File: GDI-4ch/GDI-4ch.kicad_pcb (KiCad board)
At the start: 4 copper layers, 380.4 x 234.8 mm, 165 parts, among them J14 CONN_01X03, J15 CONN_01X01, J3 CONN_02X08, J4 CONN_02X08, J7 CONN_01X03, P1 368255-2, Q1 BUK9230-100B, Q10 BUK9230-100B, Q11 BUK9230-100B, Q12 BUK9230-100B, Q2 BUK9230-100B, Q3 BUK9230-100B, Q4 BUK9230-100B, Q5 BUK9230-100B, Q6 BUK9230-100B, Q7 BUK9230-100B, Q8 BUK9230-100B, Q9 BUK9230-100B, U1 MC33816, Y2 1MHz

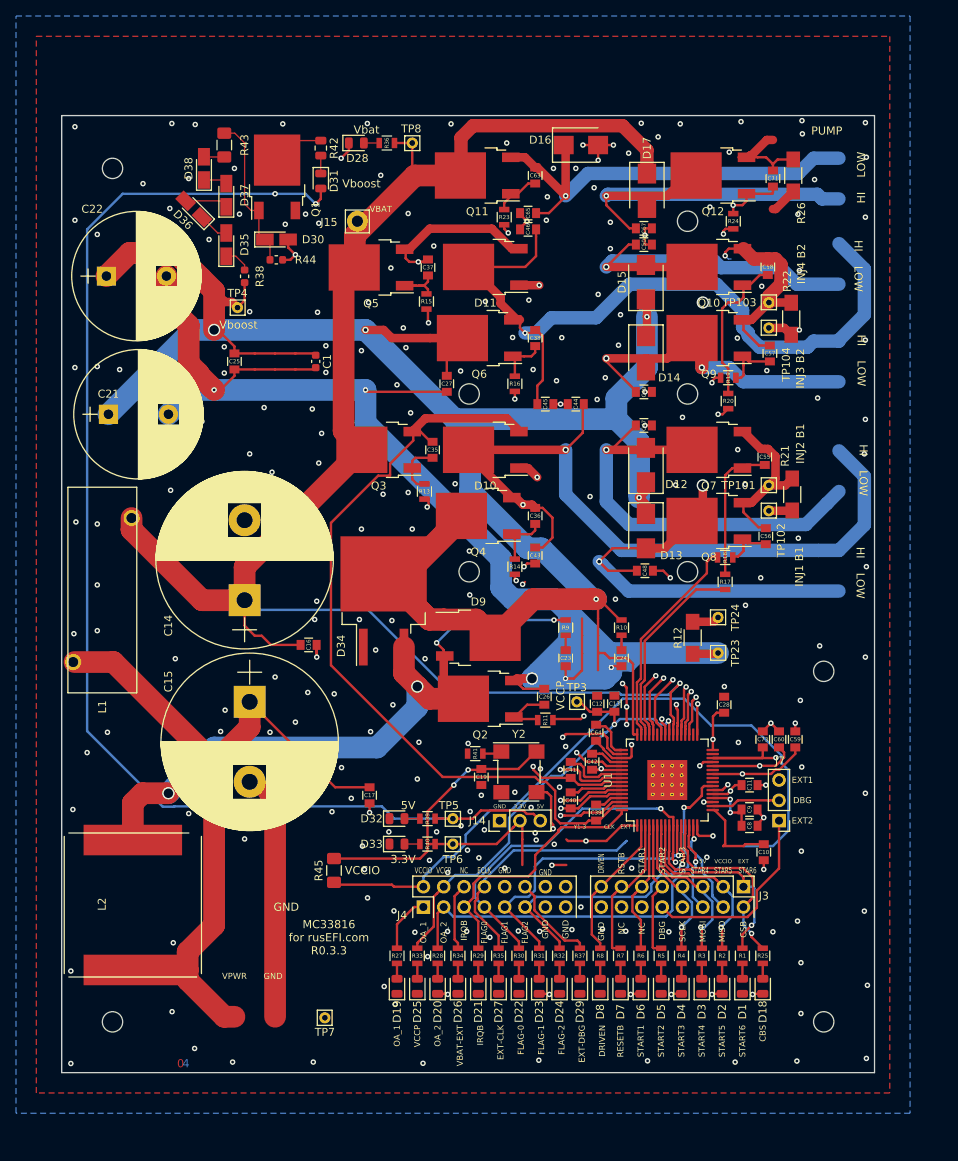
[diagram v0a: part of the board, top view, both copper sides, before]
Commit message: UPD sch
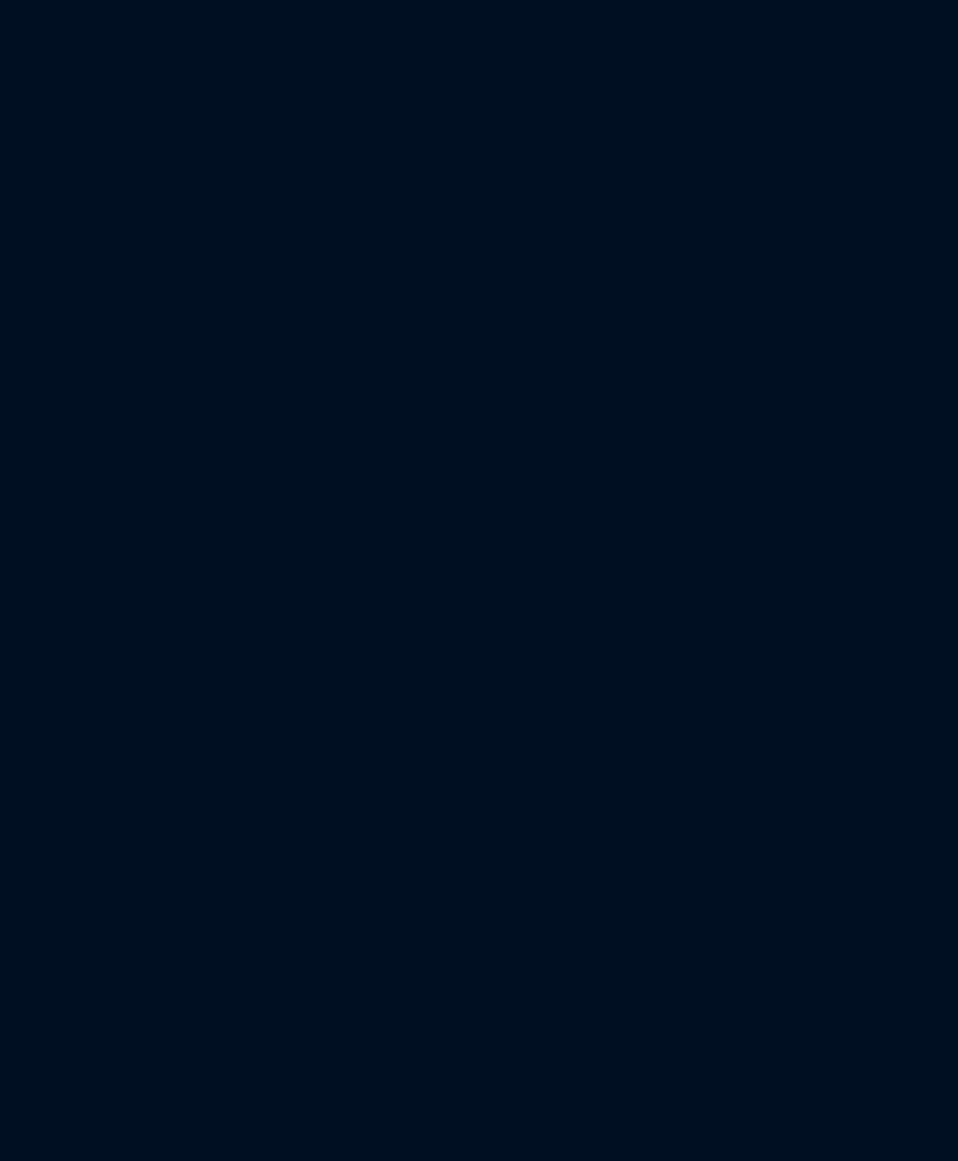
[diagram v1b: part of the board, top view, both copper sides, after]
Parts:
- removed C1: 100nF, Capacitor_SMD:C_0603_1608Metric
- removed C10, C11, C13, C8: 0.1uF, rusefi_lib:C_0805
- removed C12: 4.7uF, rusefi_lib:C_0805
- removed C14, C15: 1000uF, Capacitors_ThroughHole:CP_Radial_D22.0mm_P10.00mm_SnapIn
- removed C16, C17: 220nF, rusefi_lib:C_0805
- removed C19, C35, C36, C37, C38, C55, C56, C57, C58, C63, C71: 1000pF, rusefi_lib:C_0805
- removed C21, C22: 390uF, Capacitors_ThroughHole:CP_Radial_D16.0mm_P7.50mm
- removed C23, C24, C28, C59, C60, C73: 330pF, rusefi_lib:C_0805
- removed C25, C27: 0.22uF, rusefi_lib:C_0805
- removed C26: 470pF, rusefi_lib:C_0805
- removed C39, C40, C41, C42, C64: 0.33uF, rusefi_lib:C_0805
- removed C43, C44, C45, C46, C47, C48, C49, C50, C65, C67: 4700pF, rusefi_lib:C_0805
- removed C9: 1uF, rusefi_lib:C_0805
- removed D1, D18, D19, D2, D20, D21, D22, D23, D24, D25, D26, D27, D28, D29, D3, D31, D32, D33, D4, D5, D6, D7, D8: LED_Small, LED_SMD:LED_0805_2012Metric
- removed D10, D11: SBR10200CTL, Package_TO_SOT_SMD:TO-252-2
- removed D12, D13, D14, D15, D16, D17: STPS2H100UY, Diodes_SMD:D_SMB
- removed D30, D35, D36, D37, D38: 5.7V, Diode_SMD:D_MicroMELF_Handsoldering
- removed D34: STTH802G-TR, Package_TO_SOT_SMD:TO-263-2
- removed D9: FFD10UP20S, Package_TO_SOT_SMD:TO-252-2
- removed J14, J7: CONN_01X03, Pin_Headers:Pin_Header_Straight_1x03_Pitch2.54mm
- removed J15: CONN_01X01, Connector_Pin:Pin_D1.4mm_L8.5mm_W2.8mm_FlatFork
- removed J3, J4: CONN_02X08, Pin_Headers:Pin_Header_Straight_2x08_Pitch2.54mm
- removed L1: 6uH, rusefi_lib:744710610-Inductor
- removed L2: 10uH, rusefi_lib:IHLP6767GZER100M01
- removed Q1, Q10, Q11, Q12, Q2, Q3, Q4, Q5, Q6, Q7, Q8, Q9: BUK9230-100B, Package_TO_SOT_SMD:TO-252-2
- removed R1, R2, R25, R27, R28, R29, R3, R30, R31, R32, R33, R34, R35, R36, R37, R39, R4, R40, R5, R6, R7, R8: 1k, rusefi_lib:R_0805
- removed R10, R9: 5.1R, rusefi_lib:R_0805
- removed R11, R13, R14, R15, R16, R17, R18, R19, R20, R23, R24, R41: 10R, rusefi_lib:R_0805
- removed R12, R21, R22, R26: 0R010, Resistors_SMD:R_1206_HandSoldering
- removed R38, R44: 10k, Resistor_SMD:R_0603_1608Metric
- removed R42: 1k, Resistor_SMD:R_0805_2012Metric
- removed R43, R45: 0R010, Resistor_SMD:R_1206_3216Metric_Pad1.42x1.75mm_HandSolder
- removed TP101, TP102, TP103, TP104, TP23, TP24, TP3, TP4, TP5, TP6, TP7, TP8: CONN_01X01, Connector_Pin:Pin_D0.7mm_L6.5mm_W1.8mm_FlatFork
- removed U1: MC33816, Package_QFP:LQFP-64-1EP_10x10mm_P0.5mm_EP5x5mm_ThermalVias
- removed Y2: 1MHz, Oscillator:Oscillator_SMD_Diodes_FN-4Pin_7.0x5.0mm
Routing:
- net Vdrive: track 290.7 -> 0.00 mm, vias 5 -> 0
- net Net-(C21-Pad2): track 230.5 -> 0.00 mm, vias 6 -> 0
- net +BATT: track 214.0 -> 0.00 mm, vias 1 -> 0
- net /5V: track 177.0 -> 0.00 mm, vias 2 -> 0
- net GND: track 164.4 -> 0.00 mm, vias 277 -> 31
- net /H3: track 163.3 -> 0.00 mm, vias 2 -> 0
- net /H1: track 152.4 -> 0.00 mm, vias 3 -> 0
- net /H_PUMP: track 139.4 -> 0.00 mm, vias 2 -> 0
- net /L_PUMP: track 130.7 -> 0.00 mm, vias 2 -> 0
- net /L4: track 114.0 -> 0.00 mm, vias 2 -> 0
- net Net-(C37-Pad2): track 108.2 -> 0.00 mm, vias 3 -> 0
- net Net-(C71-Pad2): track 108.0 -> 0.00 mm, vias 1 -> 0
- net Net-(C35-Pad2): track 99.8 -> 0.00 mm
- net Net-(C60-Pad1): track 98.0 -> 0.00 mm, vias 2 -> 0
- net Net-(C10-Pad1): track 96.9 -> 0.00 mm
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- removed copper zone on B.Cu, net GND
- removed copper zone on F.Cu, net GND
- removed copper zone on In1.Cu, net GND
- removed copper zone on In2.Cu, net GND
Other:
- board size 380.4 x 234.8 mm -> 164 x 118 mm
- board text removed: "0"
- board text removed: "1"
- board text removed: "3"
- board text removed: "3.3V"
- board text removed: "4"
- board text removed: "4 layer board stackup is as follows: 0 is top min 1 oz copper (1.4 mil) min 6.7 mil prepreg FR4 1 is GND min 0.5 oz copper (0.7 mil) min 47 mil core FR4 2 is PWR min 0.5 oz copper (0.7 mil) min 6.7 mil prepreg FR4 3 is bottom min 1 oz copper (1.4 mil)"
- board text removed: "5V"
- board text removed: "CBS"
- board text removed: "CLK"
- board text removed: "CSB"
- board text removed: "DBG"
- board text removed: "DRIVEN"
- board text removed: "DRVEN"
- board text removed: "ECLK"
- board text removed: "EXT"
- board text removed: "EXT-CLK"
- board text removed: "EXT-DBG"
- board text removed: "EXT1"
- board text removed: "EXT2"
- board text removed: "FLAG-0"
- board text removed: "FLAG-1"
- board text removed: "FLAG-2"
- board text removed: "FLAG0"
- board text removed: "FLAG1"
- board text removed: "FLAG2"
- board text removed: "GND"
- board text removed: "HI LOW"
- board text removed: "INJ1 B1"
- board text removed: "INJ2 B1"
- board text removed: "INJ3 B2"
- board text removed: "INJ4 B2"
- board text removed: "IRQB"
- board text removed: "MC33816 for rusEFI.com R0.3.3"
- board text removed: "MISO"
- board text removed: "MOSI"
- board text removed: "NC"
- board text removed: "OA_1"
- board text removed: "OA_2"
- board text removed: "PUMP"
- board text removed: "RESETB"
- board text removed: "RSTB"
- board text removed: "SCLK"
- board text removed: "STAR1"
- board text removed: "STAR2"
- board text removed: "STAR3"
- board text removed: "STAR4"
- board text removed: "STAR5"
- board text removed: "STAR6"
- board text removed: "START1"
- board text removed: "START2"
- board text removed: "START3"
- board text removed: "START4"
- board text removed: "START5"
- board text removed: "START6"
- board text removed: "VBAT"
- board text removed: "VBAT-EXT"
- board text removed: "VCCIO"
- board text removed: "VCCP"
- board text removed: "VPWR"
- board text removed: "Vbat"
- board text removed: "Vboost"
- board text removed: "Y1-3"
